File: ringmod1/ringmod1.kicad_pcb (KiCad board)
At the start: 2 copper layers, 9 parts, among them J1 IN, J2 MOD, J3 OUT

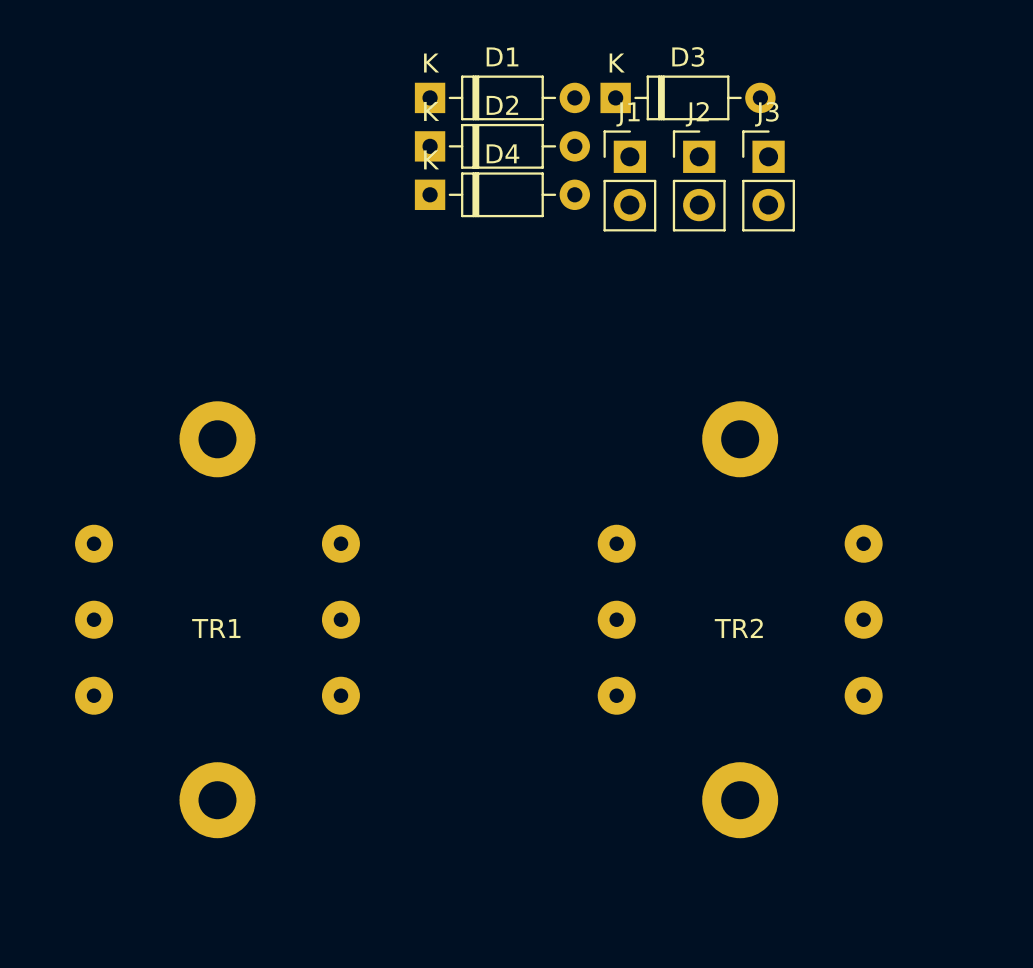
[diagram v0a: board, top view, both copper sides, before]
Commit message: initial PCB layout
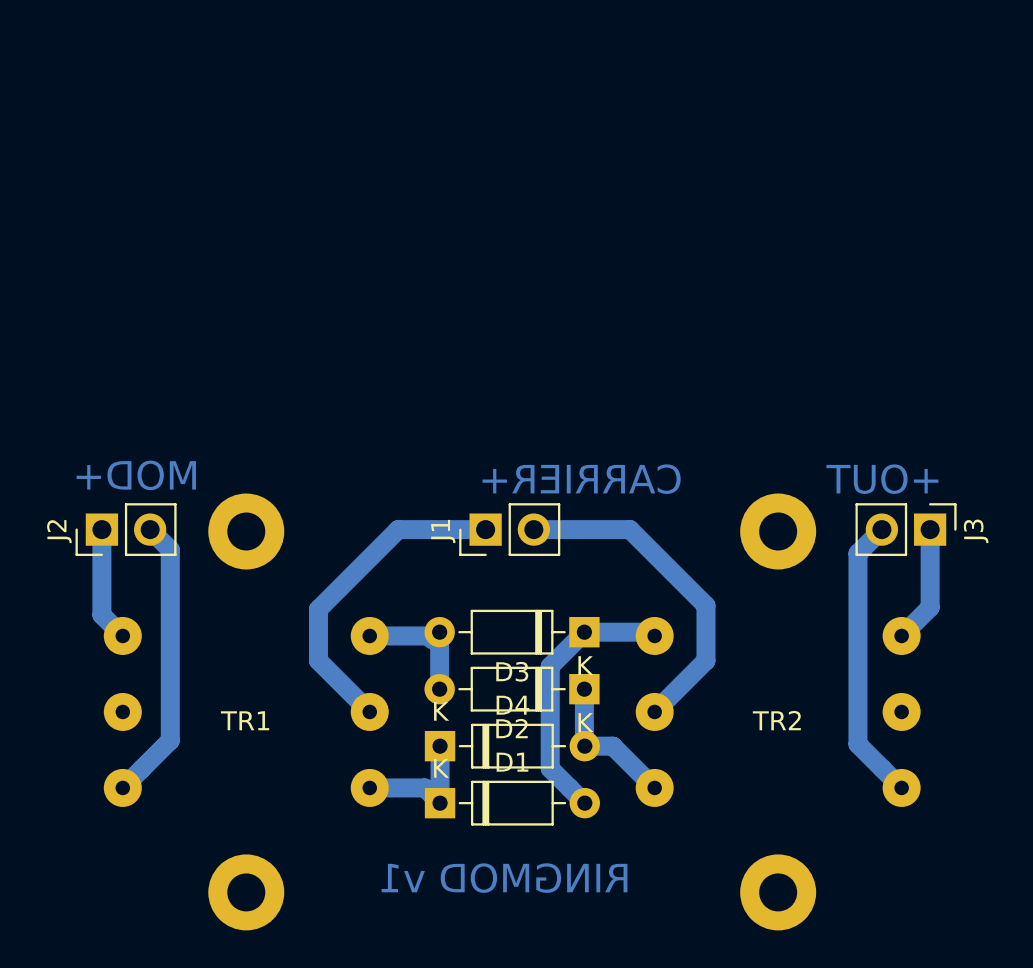
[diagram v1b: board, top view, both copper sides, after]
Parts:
- moved D1 37.1 mm to (139.6, 100.0)
- moved J2 37.1 mm to (121.8, 85.6), turned to 90 degrees
- moved D2 29.7 mm to (147.2, 94.0), turned to 180 degrees
- moved D4 29.0 mm to (139.6, 97.0)
- moved D3 28.2 mm to (147.2, 91.0), turned to 180 degrees
- moved J3 21.4 mm to (165.4, 85.6), turned to 270 degrees
- moved J1 21.0 mm to (142.0, 85.6), turned to 90 degrees
- moved TR2 5.25 mm to (157.4, 95.2)
- moved TR1 5.09 mm to (129.4, 95.2)
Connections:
- TR2 pad 4: Net-(J3-Pad2) -> Net-(J3-Pad1)
- TR2 pad 6: Net-(J3-Pad1) -> Net-(J3-Pad2)
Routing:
- net Net-(J1-Pad2): track 0.00 -> 17.4 mm
- net Net-(J1-Pad1): track 0.00 -> 17.1 mm
- net Net-(J3-Pad2): track 0.00 -> 15.1 mm
- net Net-(J2-Pad2): track 0.00 -> 15.1 mm
- net Net-(D1-Pad2): track 0.00 -> 14.3 mm
- net Net-(D2-Pad1): track 0.00 -> 7.60 mm
- net Net-(D2-Pad2): track 0.00 -> 7.33 mm
- net Net-(D1-Pad1): track 0.00 -> 7.03 mm
- net Net-(J3-Pad1): track 0.00 -> 6.22 mm
- net Net-(J2-Pad1): track 0.00 -> 6.06 mm
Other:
- net class Default: trace_width 0.25 -> 1
- net class second added: clearance 0.2, trace_width 1, via_dia 0.8, via_drill 0.4
- board text added: "+OUT"
- board text added: "CARRIER+"
- board text added: "MOD+"
- board text added: "RINGMOD v1"
